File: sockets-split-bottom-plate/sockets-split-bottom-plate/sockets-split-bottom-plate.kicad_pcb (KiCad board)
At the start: 2 copper layers, 138.1 x 85.2 mm, 0 parts

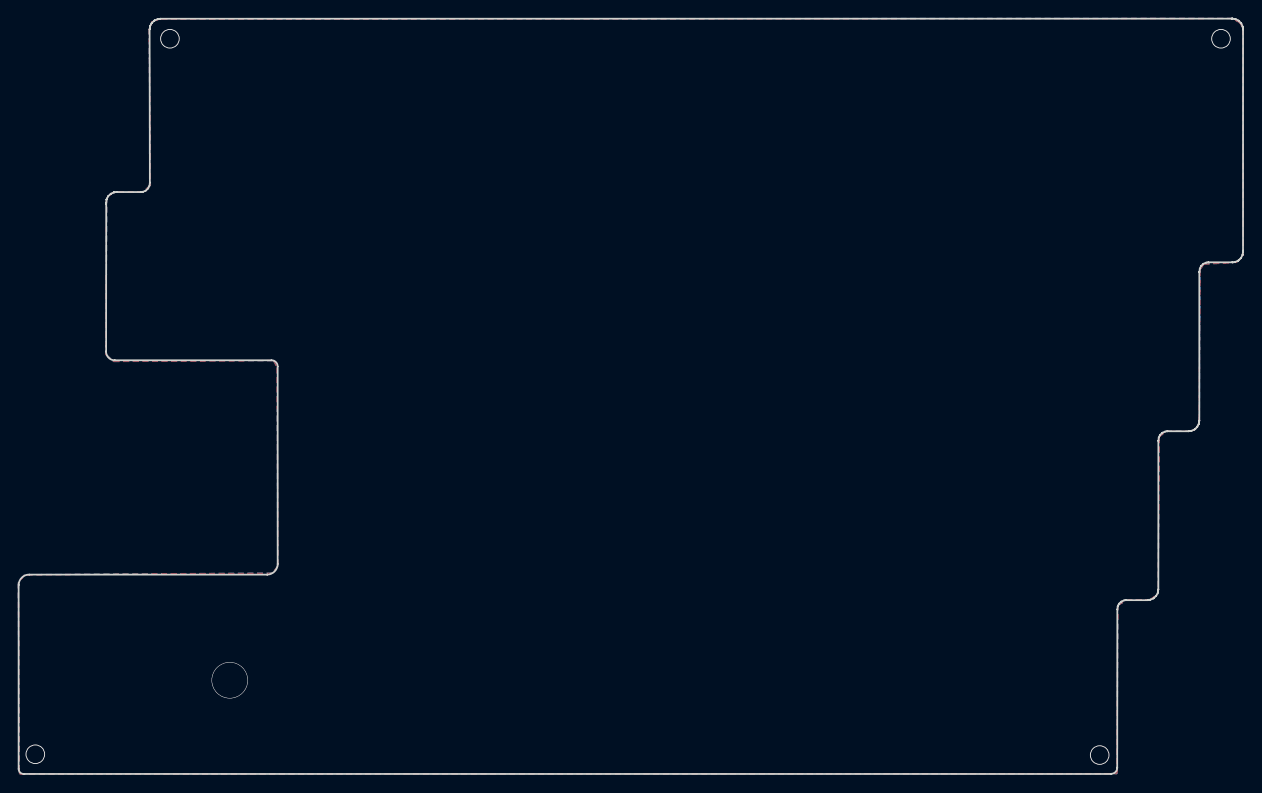
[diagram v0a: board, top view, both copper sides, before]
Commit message: Update docs
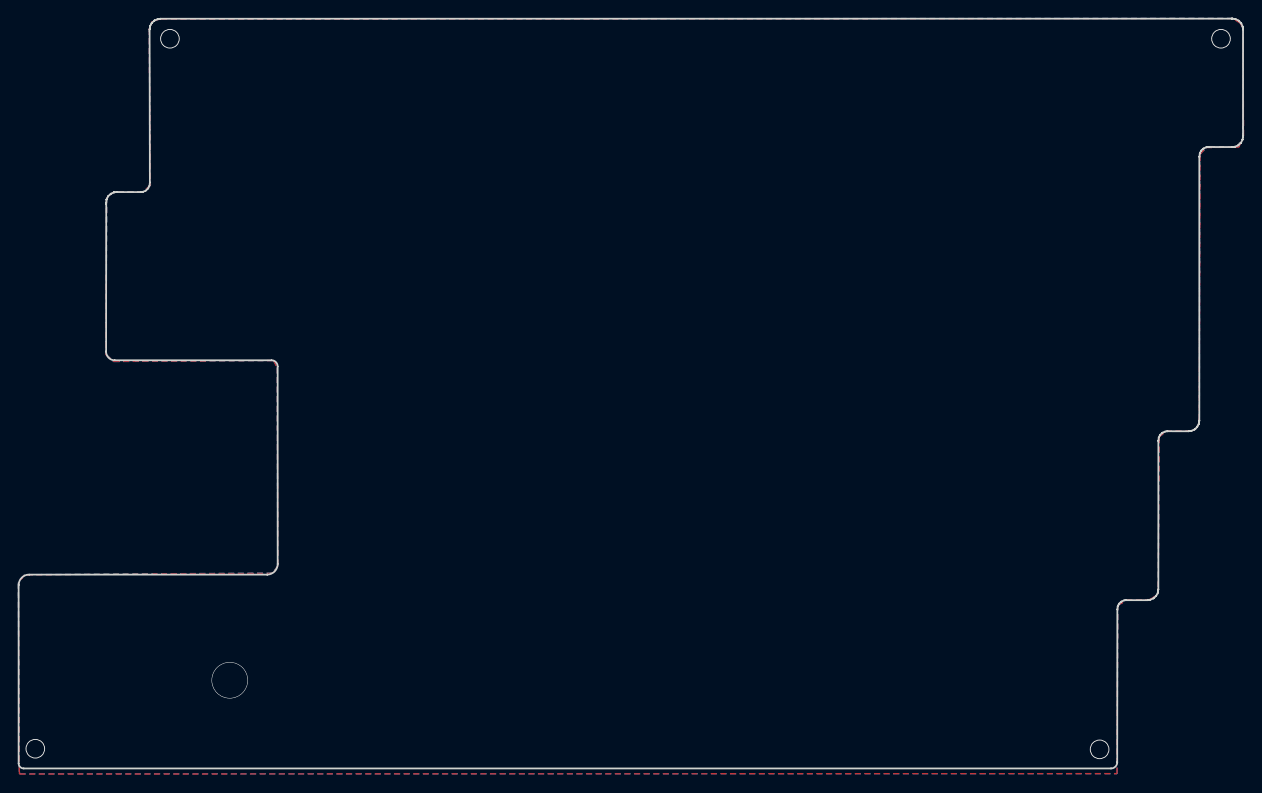
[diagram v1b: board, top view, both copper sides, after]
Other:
- board size 138.1 x 85.2 mm -> 138.1 x 84.6 mm
